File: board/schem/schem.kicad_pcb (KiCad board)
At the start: 2 copper layers, 129.8 x 66 mm, 180 parts, among them J1 no_break, J10 no_hal, J11 break2, J12 impulse, J13 hal, J14 no_temp, J15 speed, J18 adc_red1, J2 motor_out, J20 ON/OFF, J21 lamp, J3 test, J4 motor_tmp, J5 motor_tmp, J6 adc_red1, J8 POWER_IN, J9 break1, Q1 BC817, Q10 BC817, Q11 BC817, Q12 BC817, Q13 BC817, Q14 BC807, Q15 BC807, Q16 BC817, Q17 BC807, Q18 BC817, Q2 BC817, Q3 BC817, Q4 BC817, Q6 BC817, Q7 BC817, Q9 BC817, SW1 SW_Push, SW2 SW_Push, T1 CDZ44-CDI, T2 IRF4905, T3 CDZ44-CDI, T4 IRF4905, T5 CDZ44-CDI, T6 IRF4905, U1 CFPS-39-12M, U10 AP2138, U11 LD1117, U12 68u, U2 EP4CE6, U3 JTAG, U4 IS25LQ, U5 LF33CDT, U6 IS25LQ, U7 MPC3008, U8 A8498, U9 B350B

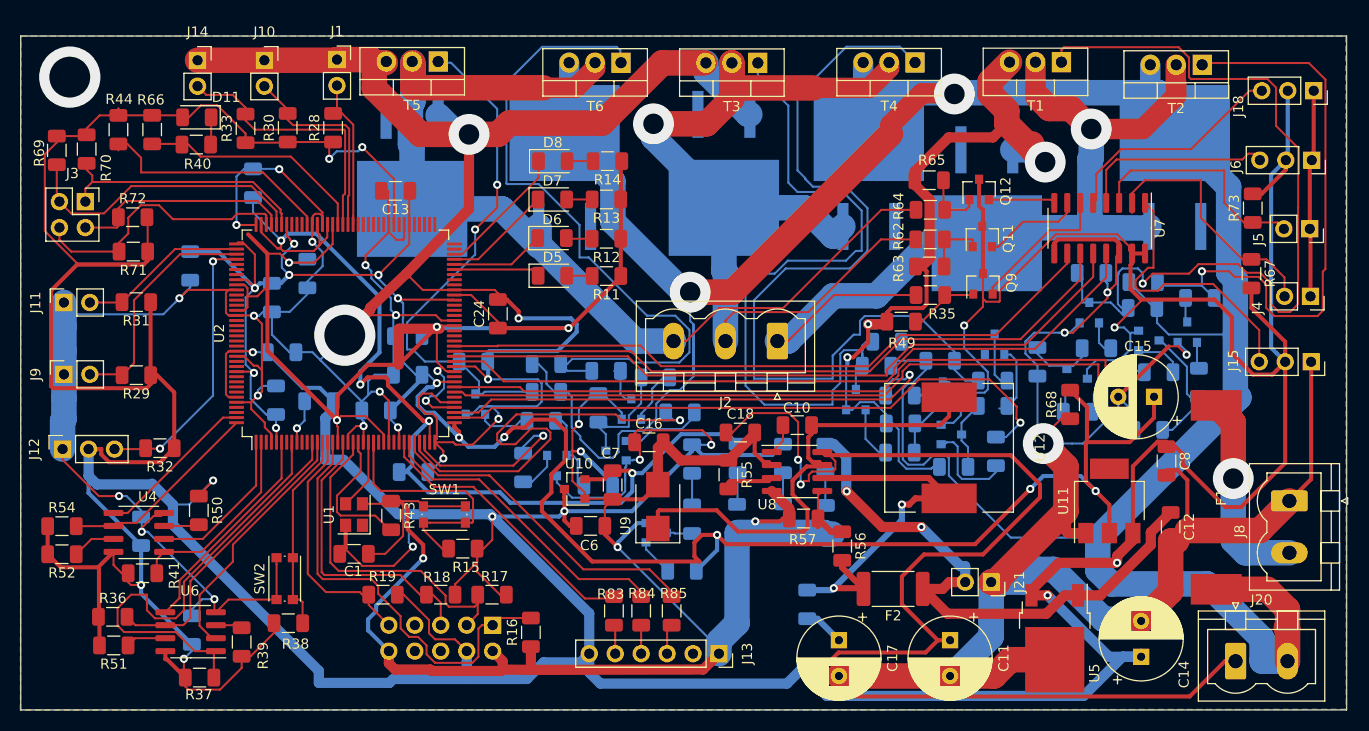
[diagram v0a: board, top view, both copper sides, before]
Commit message: minor changes
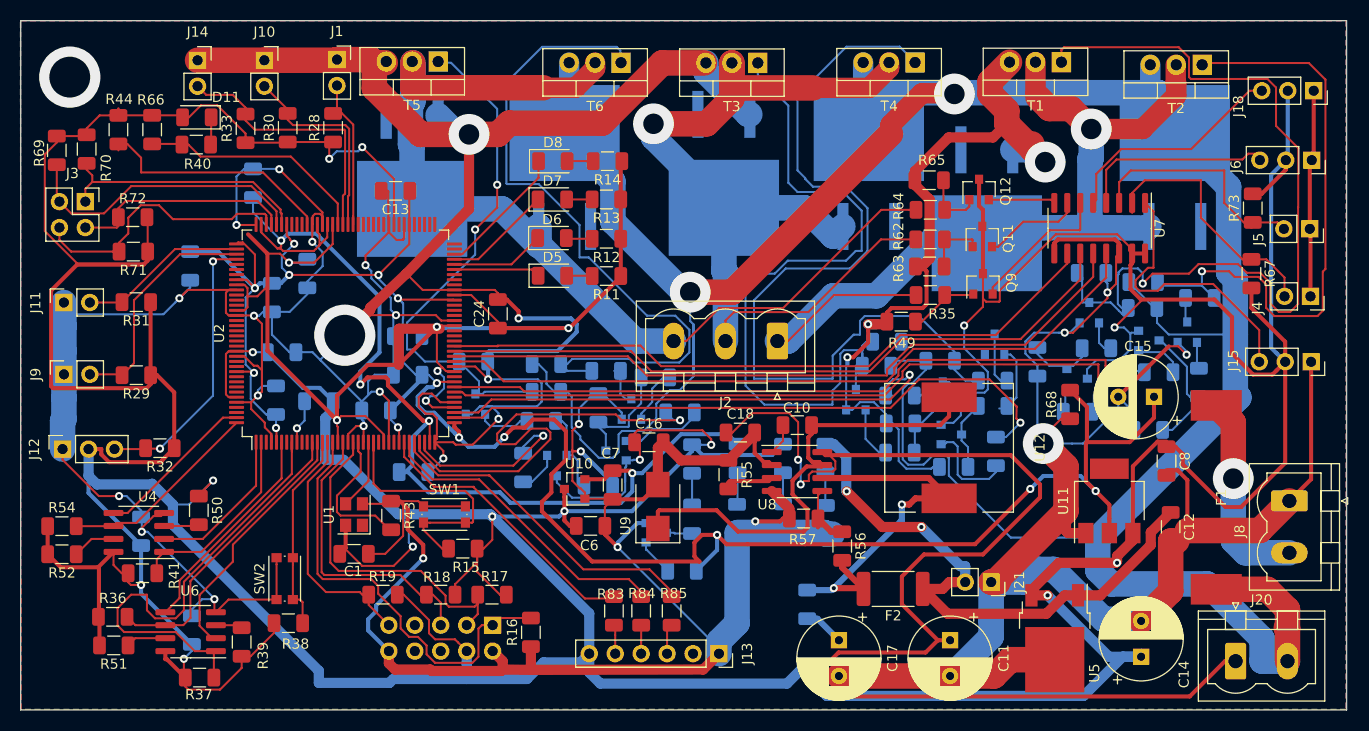
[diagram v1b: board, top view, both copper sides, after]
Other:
- board size 129.8 x 66 mm -> 129.8 x 67.5 mm
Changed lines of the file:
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@@
     (0 F.Cu signal)
     (31 B.Cu signal)
-    (32 B.Adhes user hide)
-    (33 F.Adhes user hide)
-    (34 B.Paste user hide)
-    (35 F.Paste user hide)
+    (32 B.Adhes user)
+    (33 F.Adhes user)
+    (34 B.Paste user)
+    (35 F.Paste user)
     (36 B.SilkS user)
-    (37 F.SilkS user hide)
-    (38 B.Mask user hide)
-    (39 F.Mask user hide)
-    (40 Dwgs.User user hide)
-    (41 Cmts.User user hide)
-    (42 Eco1.User user hide)
-    (43 Eco2.User user hide)
-    (44 Edge.Cuts user hide)
-    (45 Margin user hide)
-    (46 B.CrtYd user hide)
-    (47 F.CrtYd user hide)
-    (48 B.Fab user hide)
-    (49 F.Fab user hide)
+    (37 F.SilkS user)
+    (38 B.Mask user)
+    (39 F.Mask user)
+    (40 Dwgs.User user)
+    (41 Cmts.User user)
+    (42 Eco1.User user)
+    (43 Eco2.User user)
+    (44 Edge.Cuts user)
+    (45 Margin user)
+    (46 B.CrtYd user)
+    (47 F.CrtYd user)
+    (48 B.Fab user)
+    (49 F.Fab user)
   )
   (setup
@@
     )
   )
-  (gr_line (start 102 138.9836) (end 102 73) (layer Edge.Cuts) (width 0.05))
+  (gr_line (start 102 138.9836) (end 102 71.5) (layer Edge.Cuts) (width 0.05))
   (gr_line (start 231.8189 138.98298) (end 102 138.98298) (layer Edge.Cuts) (width 0.05))
-  (gr_line (start 231.8189 73) (end 231.8189 138.98298) (layer Edge.Cuts) (width 0.05))
-  (gr_line (start 102 73) (end 231.8189 73) (layer Edge.Cuts) (width 0.05))
+  (gr_line (start 231.8189 71.5) (end 231.8189 138.98298) (layer Edge.Cuts) (width 0.05))
+  (gr_line (start 102 71.5) (end 231.8189 71.5) (layer Edge.Cuts) (width 0.05))
   (via (at 106.807 77.0255) (size 6) (drill 4) (layers F.Cu B.Cu) (net 0))
   (segment (start 190.32 127.137) (end 192.7494 129.5664) (width 1) (layer F.Cu) (net 1))
@@
   (segment (start 180.003 130.051) (end 182.113 132.161) (width 0.6) (layer B.Cu) (net 76))
   (segment (start 179.0065 130.051) (end 180.003 130.051) (width 0.6) (layer B.Cu) (net 76))
-  (segment (start 192.9 117.3938) (end 192.9 118.269) (width 0.2) (layer F.Cu) (net 119))
-  (segment (start 190.91 116.279) (end 192.9 118.269) (width 0.6) (layer F.Cu) (net 119))
-  (segment (start 180.487 116.279) (end 190.91 116.279) (width 0.6) (layer F.Cu) (net 119))
-  (segment (start 189.6 118.269) (end 188.997 118.872) (width 0.6) (layer F.Cu) (net 119))
-  (segment (start 192.9 118.269) (end 189.6 118.269) (width 0.6) (layer F.Cu) (net 119))
-  (segment (start 188.997 118.872) (end 188.2775 118.872) (width 0.6) (layer F.Cu) (net 119))
-  (segment (start 188.2775 118.872) (end 188.2775 118.872) (width 0.6) (layer F.Cu) (net 119))
-  (via (at 188.2775 118.872) (size 0.8) (drill 0.4) (layers F.Cu B.Cu) (net 119))
-  (segment (start 182.4355 125.0525) (end 184.52 127.137) (width 0.6) (layer F.Cu) (net 119))
-  (segment (start 182.4355 124.339) (end 182.4355 125.0525) (width 0.6) (layer F.Cu) (net 119))
   (segment (start 121.114 130.688) (end 123.584 130.688) (width 0.2) (layer F.Cu) (net 77))
   (segment (start 123.584 130.688) (end 123.764 130.868) (width 0.2) (layer F.Cu) (net 77))
@@
   (segment (start 184.7215 112.4545) (end 186.059 113.792) (width 0.2) (layer B.Cu) (net 118))
   (segment (start 184.7215 109.601) (end 184.7215 112.4545) (width 0.2) (layer B.Cu) (net 118))
+  (segment (start 192.9 117.3938) (end 192.9 118.269) (width 0.2) (layer F.Cu) (net 119))
+  (segment (start 190.91 116.279) (end 192.9 118.269) (width 0.6) (layer F.Cu) (net 119))
+  (segment (start 180.487 116.279) (end 190.91 116.279) (width 0.6) (layer F.Cu) (net 119))
+  (segment (start 189.6 118.269) (end 188.997 118.872) (width 0.6) (layer F.Cu) (net 119))
+  (segment (start 192.9 118.269) (end 189.6 118.269) (width 0.6) (layer F.Cu) (net 119))
+  (segment (start 188.997 118.872) (end 188.2775 118.872) (width 0.6) (layer F.Cu) (net 119))
+  (segment (start 188.2775 118.872) (end 188.2775 118.872) (width 0.6) (layer F.Cu) (net 119))
+  (via (at 188.2775 118.872) (size 0.8) (drill 0.4) (layers F.Cu B.Cu) (net 119))
+  (segment (start 182.4355 125.0525) (end 184.52 127.137) (width 0.6) (layer F.Cu) (net 119))
+  (segment (start 182.4355 124.339) (end 182.4355 125.0525) (width 0.6) (layer F.Cu) (net 119))
   (segment (start 188.2775 118.872) (end 188.2775 120.396) (width 0.6) (layer B.Cu) (net 119))
   (segment (start 181.4225 127.251) (end 179.0065 127.251) (width 0.6) (layer B.Cu) (net 119))
@@
     (polygon
       (pts
-        (xy 231.8385 138.938) (xy 101.981 139.0015) (xy 102.0445 73.025) (xy 231.775 73.025)
+        (xy 231.775 138.938) (xy 102.0445 138.938) (xy 101.981 71.501) (xy 231.775 71.501)
       )
     )
@@
     (polygon
       (pts
-        (xy 231.775 138.938) (xy 101.981 139.0015) (xy 102.0445 73.025) (xy 231.775 73.025)
+        (xy 231.775 138.938) (xy 102.0445 138.938) (xy 101.981 71.501) (xy 231.775 71.501)
       )
     )
